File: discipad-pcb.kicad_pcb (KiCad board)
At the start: 2 copper layers, 76.3 x 122.8 mm, 63 parts, among them J1 AVR-ISP-6, SW0 KEYSW, SW1 KEYSW, SW10 KEYSW, SW11 KEYSW, SW12 KEYSW, SW13 KEYSW, SW14 KEYSW, SW15 KEYSW, SW16 KEYSW, SW2 KEYSW, SW3 KEYSW, SW4 KEYSW, SW5 KEYSW, SW6 KEYSW, SW7 KEYSW, SW8 KEYSW, SW9 KEYSW, U1 ATmega328P-PU, Y1 Crystal

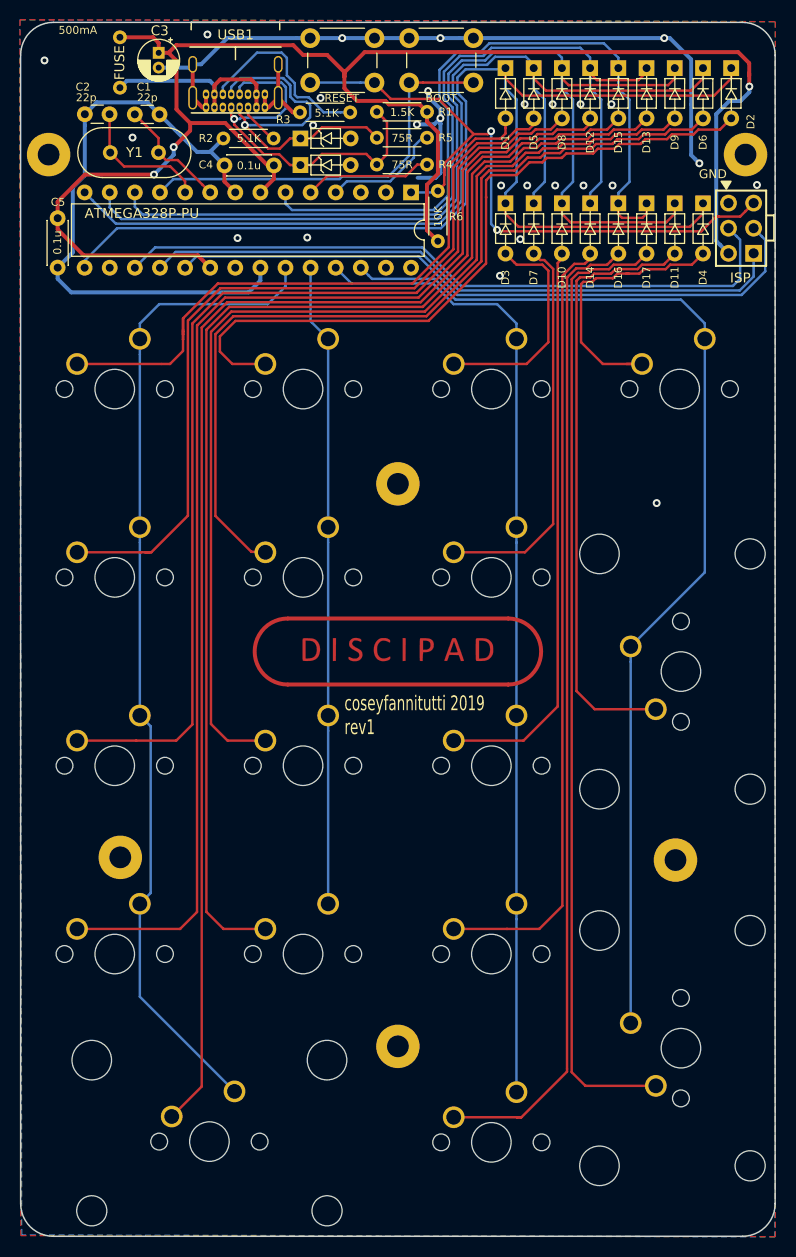
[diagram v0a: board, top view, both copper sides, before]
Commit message: version update
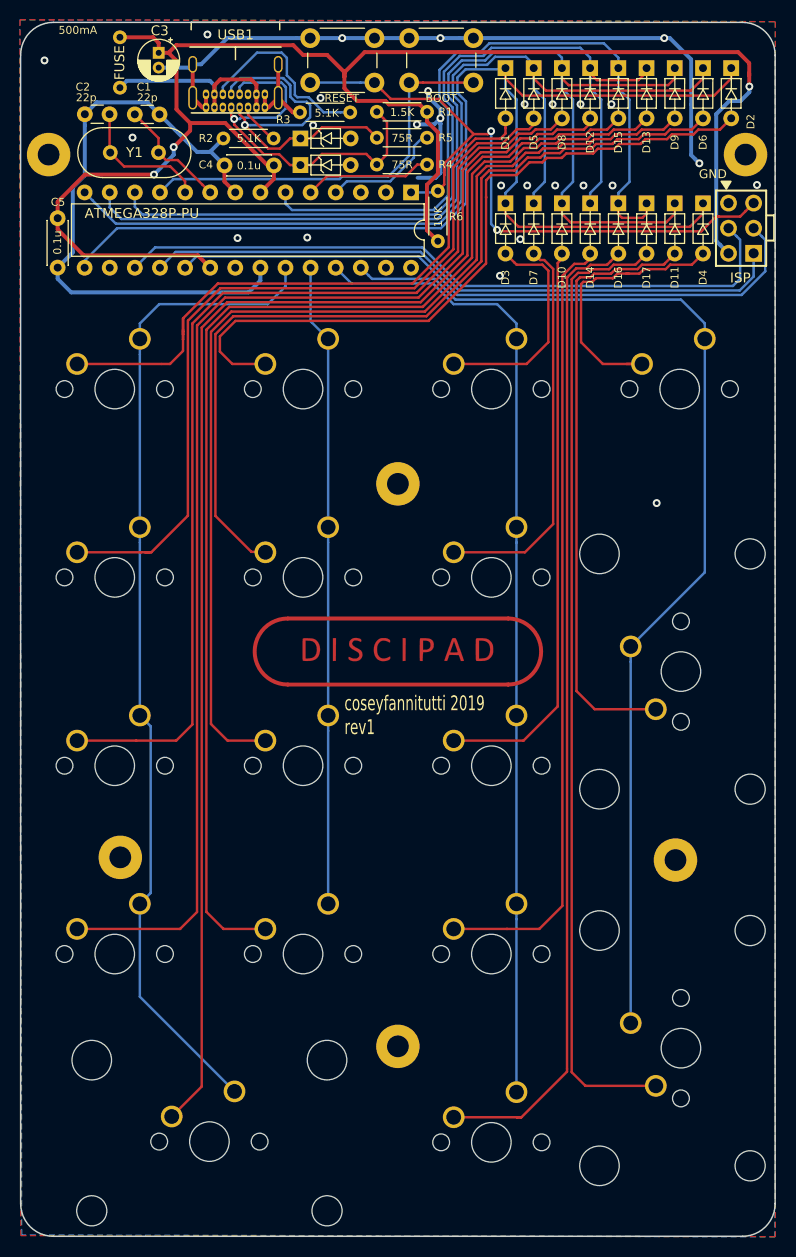
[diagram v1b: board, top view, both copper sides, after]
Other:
- net class Default removed
